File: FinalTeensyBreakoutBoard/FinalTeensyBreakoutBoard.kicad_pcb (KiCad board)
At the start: 2 copper layers, 119.4 x 109.2 mm, 40 parts, among them J1 POWER, J10 ENC3, J11 LoadCell1, J12 LoadCell2, J13 5V1, J2 MC1, J3 MC2, J4 MC3, J5 CurrSB, J6 UWB1, J7 GND1, J8 ENC1, J9 ENC2, U1 Teensy4.1, U2 MAX3284E, U3 MAX3284E, U4 MAX3284E, U5 MAX3284E, U6 MAX3284E, U7 MAX3284E

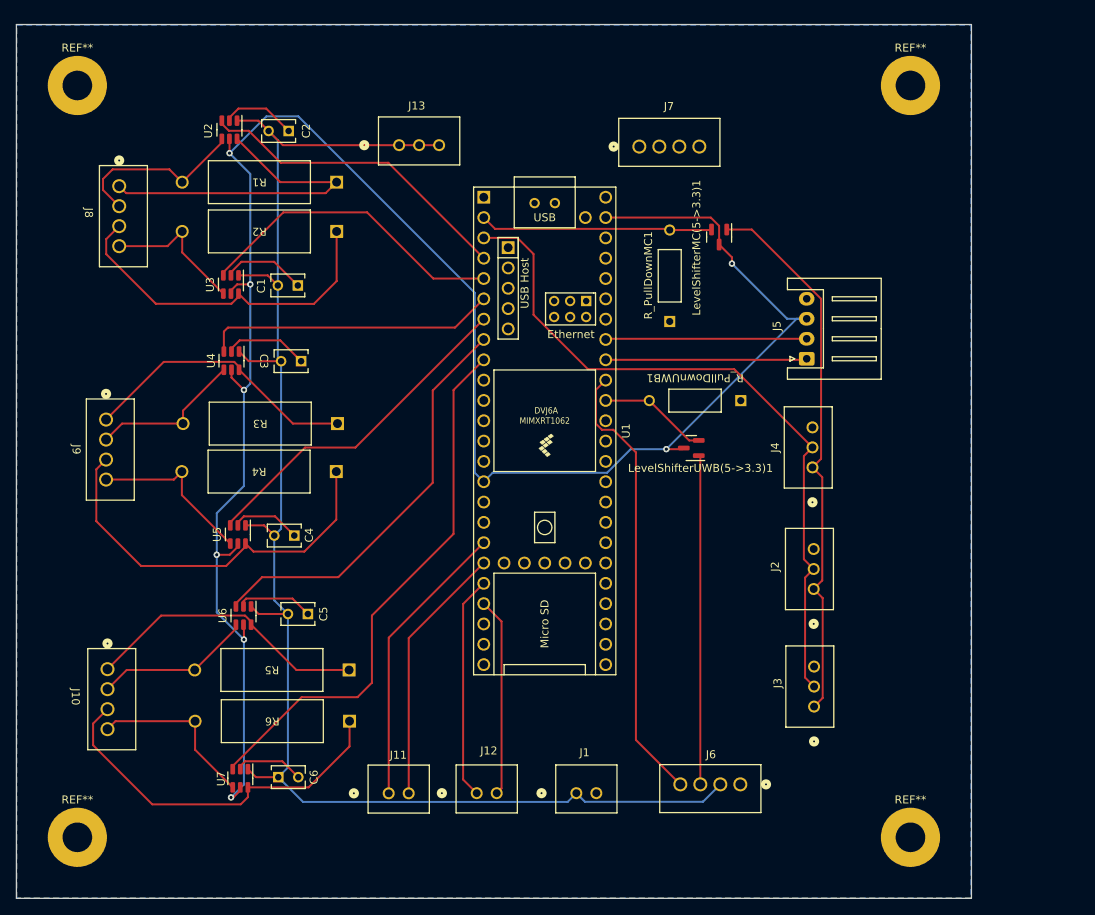
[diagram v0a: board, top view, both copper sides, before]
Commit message: Add files via upload
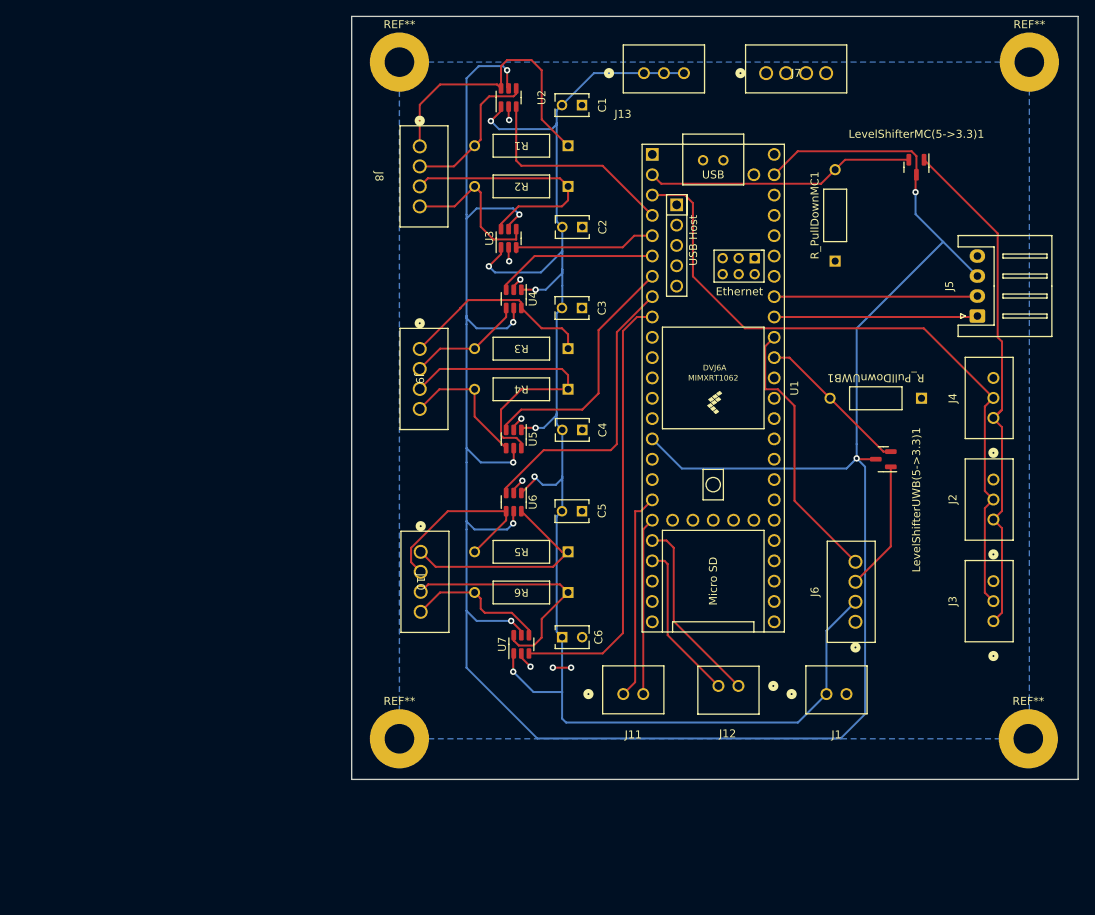
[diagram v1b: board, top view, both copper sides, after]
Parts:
- removed the REF** at (172.7, 147.3)
- removed the REF** at (68.6, 53.3)
- removed the REF** at (172.7, 53.3)
- removed the REF** at (68.6, 147.3)
- added REF**: MountingHole_3.7mm_Pad, MountingHole:MountingHole_3.7mm_Pad, F.Cu at (108.8, 50.4)
- added REF**: MountingHole_3.7mm_Pad, MountingHole:MountingHole_3.7mm_Pad, F.Cu at (187.6, 50.4)
- added REF**: MountingHole_3.7mm_Pad, MountingHole:MountingHole_3.7mm_Pad, F.Cu at (108.8, 135.0)
- added REF**: MountingHole_3.7mm_Pad, MountingHole:MountingHole_3.7mm_Pad, F.Cu at (187.5, 135.0)
- R1, R2, R3, R4, R5, R6: footprint teensy:100ohmR -> teensy:100ohmRnew
- moved C1 42.1 mm to (131.7, 55.8)
- moved J10 41.8 mm to (111.5, 111.6)
- moved J9 40.2 mm to (111.4, 86.3)
- moved C6 39.6 mm to (129.2, 122.3)
- moved U7 38.9 mm to (124.1, 123.2), turned to 90 degrees
- moved C2 38.6 mm to (131.7, 71.0)
- moved C4 38.3 mm to (131.7, 96.4)
- moved J8 37.9 mm to (111.4, 61.0)
- moved U6 36.6 mm to (123.1, 105.4)
- moved C5 36.6 mm to (131.7, 106.6)
- moved U5 36.5 mm to (123.1, 97.5)
- moved U4 36.1 mm to (123.1, 80.0)
- moved C3 35.7 mm to (131.7, 81.2)
- moved J12 35.4 mm to (151.2, 128.4), turned to 180 degrees
- moved U3 35.2 mm to (122.5, 72.4), turned to 90 degrees
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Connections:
- U1 pad 13: /MOSI -> unconnected-(U1-11_MOSI_CTX1-Pad13)
- U1 pad 14: /MISO -> unconnected-(U1-12_MISO_MQSL-Pad14)
- U1 pad 35: /SCK -> unconnected-(U1-13_SCK_LED-Pad35)
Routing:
- net +3.3V: track 249.8 -> 311.9 mm
- net GND: track 57.6 -> 13.3 mm, vias 0 -> 8
- net /RX1: track 41.2 -> 16.2 mm
- net /TX1: track 56.2 -> 34.1 mm
- net /EncB: track 39.5 -> 18.2 mm
- net /Enc1A: track 36.7 -> 20.4 mm
- net /B2: track 47.2 -> 31.1 mm
- net /Enc2A: track 51.8 -> 37.0 mm
- net /EncA: track 40.1 -> 26.6 mm
- net /Enc2B: track 68.3 -> 55.0 mm
- net /B: track 44.2 -> 31.4 mm
- net /B1: track 50.0 -> 38.3 mm
- net /Enc1B: track 42.6 -> 31.2 mm
- net /WDAT1: track 32.7 -> 22.2 mm
- net /A1: track 35.3 -> 25.0 mm
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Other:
- board size 119.4 x 109.2 mm -> 90.8 x 95.4 mm
